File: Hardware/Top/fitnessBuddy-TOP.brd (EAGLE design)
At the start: 38 x 38 mm, 50 parts, among them SW3 SWITCH.MOM, SW4 SWITCH.MOM, U1 NRF52832_MODULE_MDBT42, U2 FT231XS

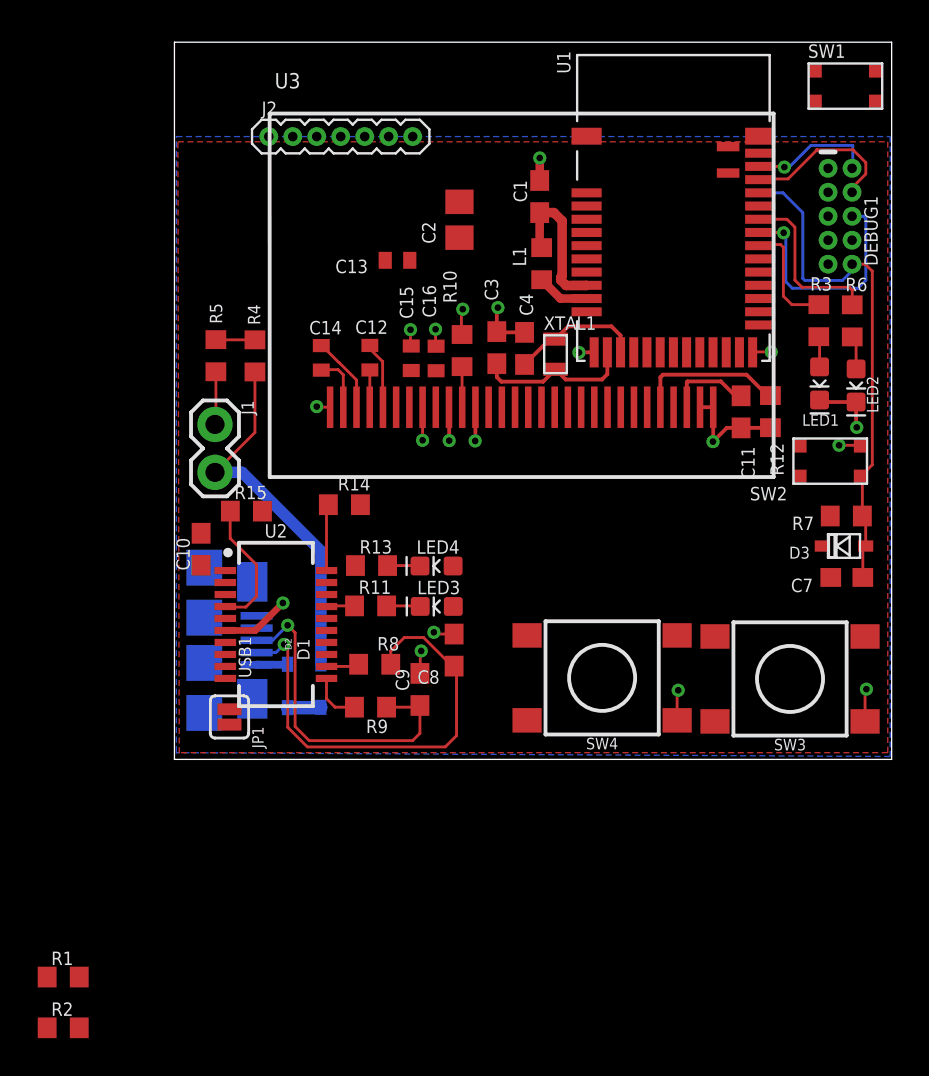
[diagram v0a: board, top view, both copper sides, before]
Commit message: finished halfway through take 007. organized board/ connected airwires
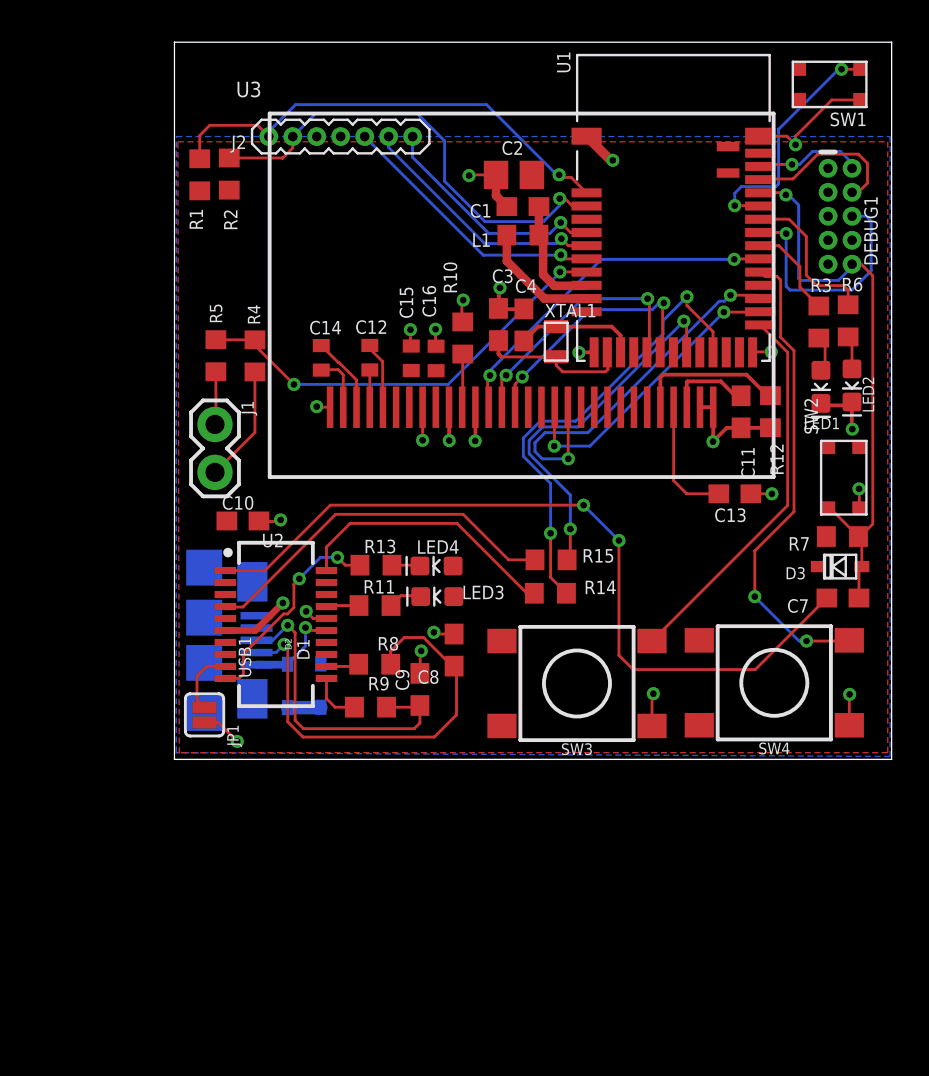
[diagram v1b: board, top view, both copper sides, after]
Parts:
- C13: device LinnesLab-Passives:C0402 -> LinnesLab-Passives:C0603
- moved R2 46.1 mm to (2.91, 31.0), turned to 270 degrees
- moved R1 43.1 mm to (1.34, 31.0), turned to 270 degrees
- moved C13 21.7 mm to (29.7, 14.1), turned to 180 degrees
- moved R15 16.3 mm to (20.0, 10.6)
- moved R14 11.9 mm to (19.9, 8.80)
- moved SW3 11.3 mm to (21.3, 4.02)
- moved SW4 9.13 mm to (31.8, 4.06)
- moved C2 3.74 mm to (18.0, 31.0), turned to 0 degrees
- moved C10 2.68 mm to (3.63, 12.6), turned to 180 degrees
- moved L1 1.81 mm to (18.5, 27.8), turned to 0 degrees
- moved JP1 1.33 mm to (1.60, 2.36)
- moved C4 1.25 mm to (18.5, 23.0)
- moved C3 1.23 mm to (17.2, 23.0)
- moved SW2 1.14 mm to (35.5, 14.9), turned to 90 degrees
- moved D3 1.11 mm to (35.3, 10.2)
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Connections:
- removed net !DTR: U2.1
- removed net A4/BATT: R4.1, R5.2, U1.5
- removed net A6/TIA: J2.6, U1.7
- removed net A7/PPG: J2.7, U1.8
- removed net D29/LED.CTRL: J2.5, U1.6
- new net A4/PPG: J2.7, U1.5
- new net A5/TIA: J2.6, U1.6
- new net A7/BATT: R4.1, R5.2, U1.8
- new net D30/LED.CTRL: J2.5, U1.7
- net DTR: now also U2.1
- net GND: no longer SW3.B2, SW4.B2
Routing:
- net DTR: track 0.00 -> 42.0 mm, vias 0 -> 2
- net SDA: track 0.00 -> 25.0 mm, vias 0 -> 1
- net SCL: track 0.00 -> 24.9 mm, vias 0 -> 1
- net RXD.NRF: track 0.00 -> 24.9 mm, vias 0 -> 2
- net D15/SW2: track 0.76 -> 25.3 mm, vias 0 -> 2
- net A7/BATT: track 0.00 -> 23.3 mm, vias 0 -> 2
- net MOSI: track 0.00 -> 20.4 mm, vias 0 -> 2
- net D11/SW1: track 0.03 -> 20.3 mm
- net TXD.NRF: track 0.00 -> 19.8 mm, vias 0 -> 2
- net D16/CS.OLED: track 0.00 -> 18.8 mm, vias 0 -> 2
- net SCK: track 0.00 -> 15.9 mm, vias 0 -> 2
- net GND: track 37.9 -> 53.7 mm, vias 19 -> 25
- net D30/LED.CTRL: track 0.00 -> 14.5 mm, vias 0 -> 1
- net D3/RESET.OLED: track 0.00 -> 13.9 mm, vias 0 -> 2
- net D4/DC.OLED: track 0.00 -> 13.6 mm, vias 0 -> 2
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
